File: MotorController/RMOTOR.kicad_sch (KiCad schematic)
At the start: 18 parts

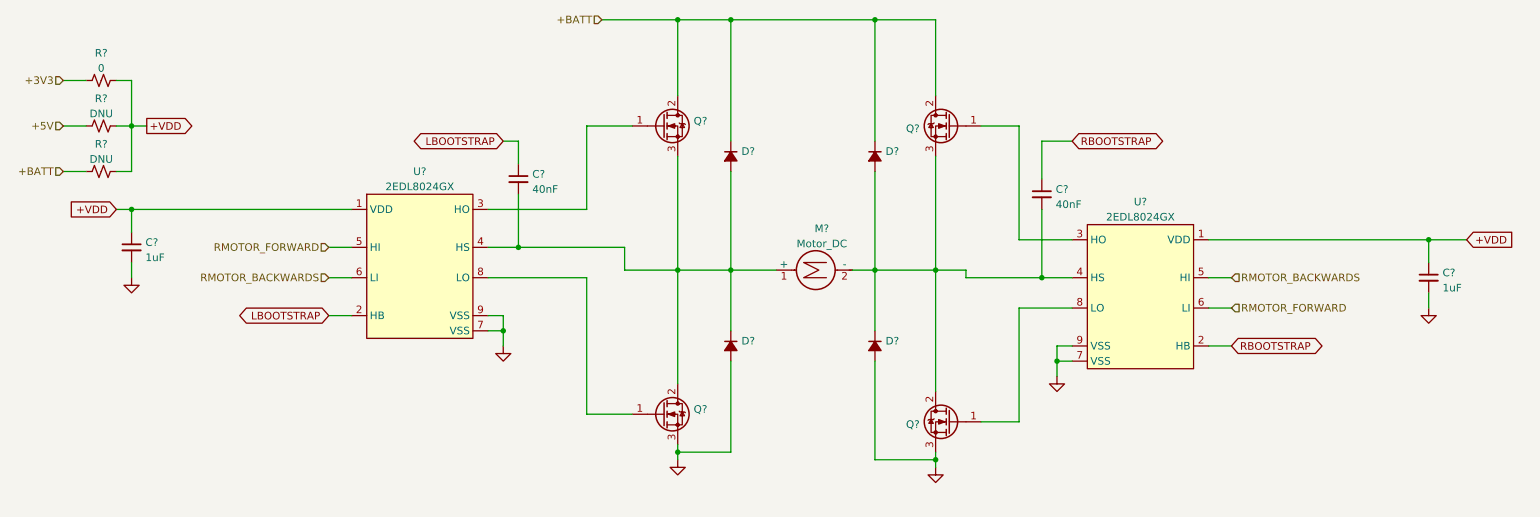
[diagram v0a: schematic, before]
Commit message: More updates
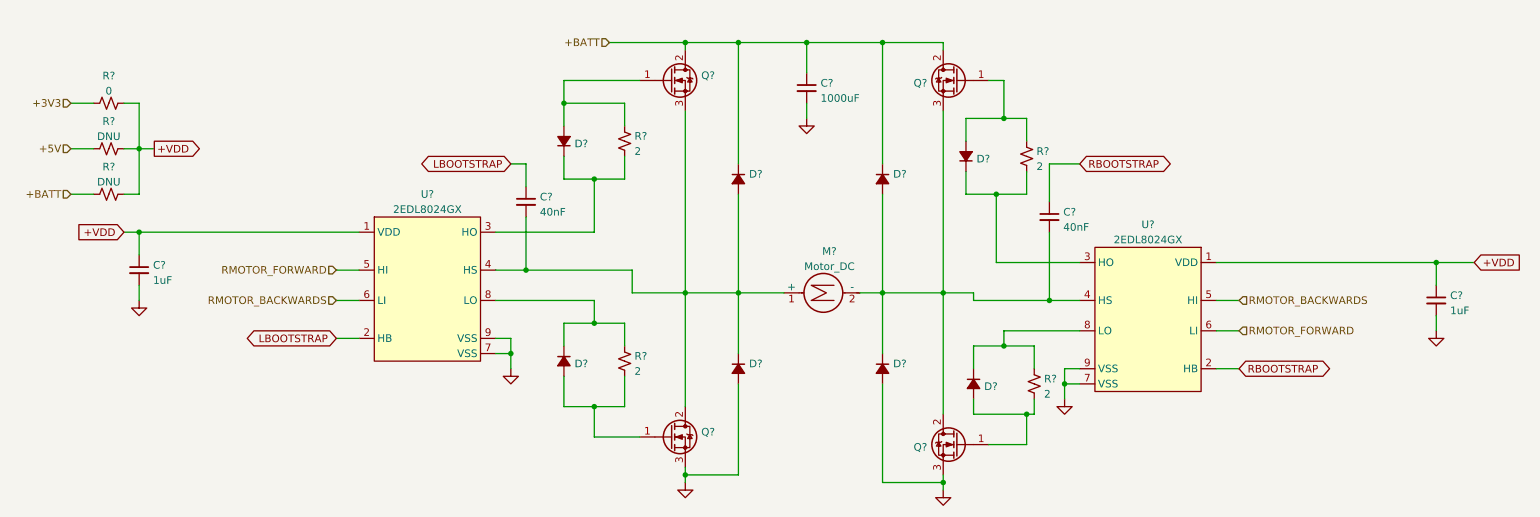
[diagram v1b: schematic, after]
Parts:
- removed C? (x2): 40nF, symbol Device:C_Small
- removed C? (x2): 1uF, symbol Device:C_Small
- removed D? (x4): D_Small_Filled, symbol Device:D_Small_Filled
- removed M?: Motor_DC, symbol Motor:Motor_DC
- removed Q? (x4): Q_NMOS_GDS, symbol Device:Q_NMOS_GDS
- removed R? (x2): DNU, symbol Device:R_Small_US
- removed R?: 0, symbol Device:R_Small_US
- removed U? (x2): 2EDL8024GX, symbol ProjectSymbols:2EDL8024GX
- added C? (x2): 40nF, symbol Device:C_Small
- added C? (x2): 1uF, symbol Device:C_Small
- added C?: 1000uF, symbol Device:C_Small
- added D? (x8): D_Small_Filled, symbol Device:D_Small_Filled
- added M?: Motor_DC, symbol Motor:Motor_DC
- added Q? (x4): Q_NMOS_GDS, symbol Device:Q_NMOS_GDS
- added R? (x4): 2, symbol Device:R_Small_US
- added R? (x2): DNU, symbol Device:R_Small_US
- added R?: 0, symbol Device:R_Small_US
- added U? (x2): 2EDL8024GX, symbol ProjectSymbols:2EDL8024GX
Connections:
- net +3V3: now also R?.1
- net +5V: now also R?.1
- net +BATT: now also C?.1, D?.1 (K), D?.1 (K), Q?.2 (D), Q?.2 (D), R?.1
- net +VDD: now also C?.1, C?.1, R?.2, R?.2, R?.2, U?.1 (VDD), U?.1 (VDD)
- net GND: now also C?.2, C?.2, C?.2, D?.2 (A), D?.2 (A), Q?.3 (S), Q?.3 (S), U?.7 (VSS), U?.7 (VSS), U?.9 (VSS), U?.9 (VSS)
- net LBOOTSTRAP: now also C?.1, U?.2 (HB)
- net RBOOTSTRAP: now also C?.1, U?.2 (HB)
- net RMOTOR_BACKWARDS: now also U?.5 (HI), U?.6 (LI)
- net RMOTOR_FORWARD: now also U?.5 (HI), U?.6 (LI)
- new net: C?.2, D?.1 (K), D?.2 (A), M?.1 (+), Q?.2 (D), Q?.3 (S), U?.4 (HS)
- new net: D?.2 (A), Q?.1 (G), R?.1 (x2)
- new net: D?.1 (K), R?.2, U?.3 (HO) (x2)
- new net: D?.2 (A), Q?.1 (G), R?.2 (x2)
- new net: C?.2, D?.1 (K), D?.2 (A), M?.2 (-), Q?.2 (D), Q?.3 (S), U?.4 (HS)
- new net: D?.1 (K), R?.1, U?.8 (LO) (x2)
